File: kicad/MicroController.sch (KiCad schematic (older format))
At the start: 6 parts, among them P3 MIKROPROG, U1 LM324, U2 PIC16F1779

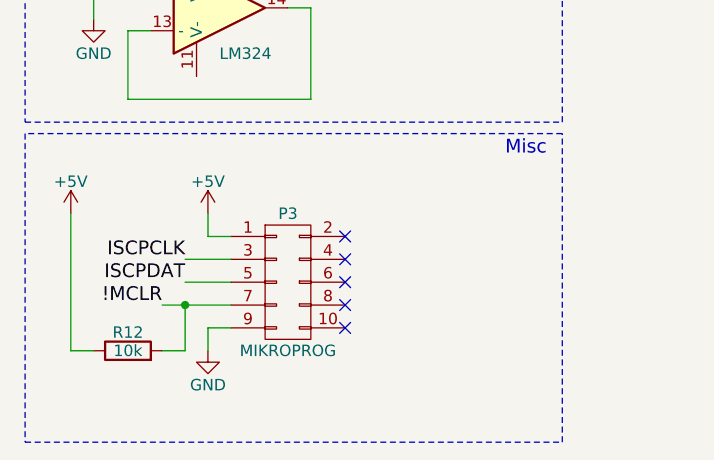
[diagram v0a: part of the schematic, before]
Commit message: Edited schematics
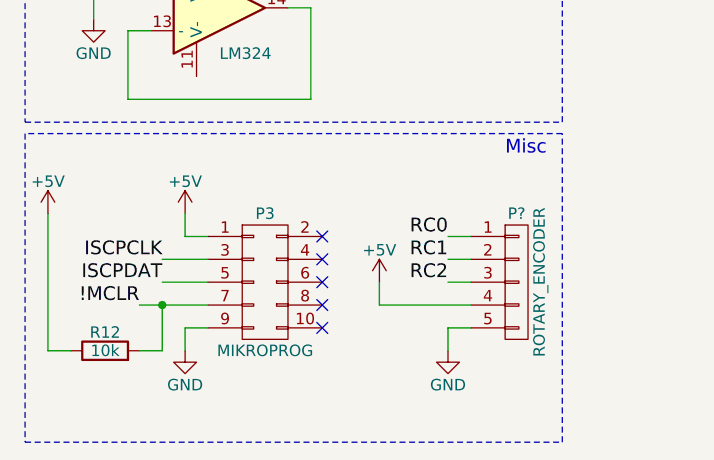
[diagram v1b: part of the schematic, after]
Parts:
- added P?: ROTARY_ENCODER, symbol CONN_01X05
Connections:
- net +5V: now also P?.4 (P4)
- net GND: now also P?.5 (P5)
- net RC0: now also P?.1 (P1)
- net RC1: now also P?.2 (P2)
- net RC2: now also P?.3 (P3)
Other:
- moved on the sheet: P3, R12
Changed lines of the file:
@@
 L CONN_02X05 P3
 U 1 1 59B71C9D
-P 1700 7000
-F 0 "P3" H 1700 7300 50  0000 C CNN
-F 1 "MIKROPROG" H 1700 6700 50  0000 C CNN
-F 2 "" H 1700 5800 50  0001 C CNN
-F 3 "" H 1700 5800 50  0000 C CNN
-	1    1700 7000
+P 1600 7000
+F 0 "P3" H 1600 7300 50  0000 C CNN
+F 1 "MIKROPROG" H 1600 6700 50  0000 C CNN
+F 2 "" H 1600 5800 50  0001 C CNN
+F 3 "" H 1600 5800 50  0000 C CNN
+	1    1600 7000
 	1    0    0    -1
 $EndComp
@@
 L +5V #PWR06
 U 1 1 59B71CA4
-P 750 6700
-F 0 "#PWR06" H 750 6550 50  0001 C CNN
-F 1 "+5V" H 750 6840 50  0000 C CNN
-F 2 "" H 750 6700 50  0000 C CNN
-F 3 "" H 750 6700 50  0000 C CNN
-	1    750  6700
-	1    0    0    -1
-$EndComp
-Wire Wire Line
-	1350 6700 1350 6800
-Wire Wire Line
-	1350 6800 1450 6800
-Text Label 1250 6900 2    60   ~ 0
+P 650 6700
+F 0 "#PWR06" H 650 6550 50  0001 C CNN
+F 1 "+5V" H 650 6840 50  0000 C CNN
+F 2 "" H 650 6700 50  0000 C CNN
+F 3 "" H 650 6700 50  0000 C CNN
+	1    650  6700
+	1    0    0    -1
+$EndComp
+Wire Wire Line
+	1250 6700 1250 6800
+Wire Wire Line
+	1250 6800 1350 6800
+Text Label 1150 6900 2    60   ~ 0
 ISCPCLK
-Text Label 1250 7000 2    60   ~ 0
+Text Label 1150 7000 2    60   ~ 0
 ISCPDAT
-Text Label 1150 7100 2    60   ~ 0
+Text Label 1050 7100 2    60   ~ 0
 !MCLR
 Wire Wire Line
-	1250 6900 1450 6900
-Wire Wire Line
-	1250 7000 1450 7000
-Wire Wire Line
-	1150 7100 1450 7100
-NoConn ~ 1950 6800
-NoConn ~ 1950 6900
-NoConn ~ 1950 7000
-NoConn ~ 1950 7100
-NoConn ~ 1950 7200
+	1150 6900 1350 6900
+Wire Wire Line
+	1150 7000 1350 7000
+Wire Wire Line
+	1050 7100 1350 7100
+NoConn ~ 1850 6800
+NoConn ~ 1850 6900
+NoConn ~ 1850 7000
+NoConn ~ 1850 7100
+NoConn ~ 1850 7200
 $Comp
 L GND #PWR07
 U 1 1 59B71CB7
-P 1350 7300
-F 0 "#PWR07" H 1350 7050 50  0001 C CNN
-F 1 "GND" H 1350 7150 50  0000 C CNN
-F 2 "" H 1350 7300 50  0000 C CNN
-F 3 "" H 1350 7300 50  0000 C CNN
-	1    1350 7300
-	1    0    0    -1
-$EndComp
-Wire Wire Line
-	1350 7200 1450 7200
+P 1250 7300
+F 0 "#PWR07" H 1250 7050 50  0001 C CNN
+F 1 "GND" H 1250 7150 50  0000 C CNN
+F 2 "" H 1250 7300 50  0000 C CNN
+F 3 "" H 1250 7300 50  0000 C CNN
+	1    1250 7300
+	1    0    0    -1
+$EndComp
+Wire Wire Line
+	1250 7200 1350 7200
 Text HLabel 1650 900  0    60   Input ~ 0
 5V
@@
 L R R12
 U 1 1 59B74780
-P 1000 7300
-F 0 "R12" V 1080 7300 50  0000 C CNN
-F 1 "10k" V 1000 7300 50  0000 C CNN
-F 2 "Resistors_SMD:R_0805_HandSoldering" V 930 7300 50  0001 C CNN
-F 3 "" H 1000 7300 50  0000 C CNN
-	1    1000 7300
+P 900 7300
+F 0 "R12" V 980 7300 50  0000 C CNN
+F 1 "10k" V 900 7300 50  0000 C CNN
+F 2 "Resistors_SMD:R_0805_HandSoldering" V 830 7300 50  0001 C CNN
+F 3 "" H 900 7300 50  0000 C CNN
+	1    900  7300
 	0    -1   -1   0
 $EndComp
 Wire Wire Line
-	1250 7100 1250 7300
-Connection ~ 1250 7100
+	1150 7100 1150 7300
+Connection ~ 1150 7100
 Wire Wire Line
 	1100 5100 1000 5100
@@
 	850  5700 1100 5700
 Wire Wire Line
-	1250 7300 1150 7300
-Wire Wire Line
-	850  7300 750  7300
-Wire Wire Line
-	750  7300 750  6700
+	1150 7300 1050 7300
+Wire Wire Line
+	750  7300 650  7300
+Wire Wire Line
+	650  7300 650  6700
 $Comp
 L +5V #PWR016
 U 1 1 59B75D07
-P 1350 6700
-F 0 "#PWR016" H 1350 6550 50  0001 C CNN
-F 1 "+5V" H 1350 6840 50  0000 C CNN
-F 2 "" H 1350 6700 50  0000 C CNN
-F 3 "" H 1350 6700 50  0000 C CNN
-	1    1350 6700
-	1    0    0    -1
-$EndComp
-Wire Wire Line
-	1350 7300 1350 7200
+P 1250 6700
+F 0 "#PWR016" H 1250 6550 50  0001 C CNN
+F 1 "+5V" H 1250 6840 50  0000 C CNN
+F 2 "" H 1250 6700 50  0000 C CNN
+F 3 "" H 1250 6700 50  0000 C CNN
+	1    1250 6700
+	1    0    0    -1
+$EndComp
+Wire Wire Line
+	1250 7300 1250 7200
 Wire Wire Line
 	3350 950  3250 950
@@
 Text Notes 4650 700  0    60   ~ 0
 MICROCONTROLLER
+$Comp
+L CONN_01X05 P?
+U 1 1 59B8D999
+P 2700 7000
+F 0 "P?" H 2700 7300 50  0000 C CNN
+F 1 "ROTARY_ENCODER" V 2800 7000 50  0000 C CNN
+F 2 "" H 2700 7000 50  0000 C CNN
+F 3 "" H 2700 7000 50  0000 C CNN
+	1    2700 7000
+	1    0    0    -1
+$EndComp
+$Comp
+L GND #PWR?
+U 1 1 59B8DA9A
+P 2400 7300
+F 0 "#PWR?" H 2400 7050 50  0001 C CNN
+F 1 "GND" H 2400 7150 50  0000 C CNN
+F 2 "" H 2400 7300 50  0000 C CNN
+F 3 "" H 2400 7300 50  0000 C CNN
+	1    2400 7300
+	1    0    0    -1
+$EndComp
+Wire Wire Line
+	2400 7300 2400 7200
+Wire Wire Line
+	2400 7200 2500 7200
+Text Label 2400 6800 2    60   ~ 0
+RC0
+Text Label 2400 6900 2    60   ~ 0
+RC1
+Text Label 2400 7000 2    60   ~ 0
+RC2
+Wire Wire Line
+	2400 6800 2500 6800
+Wire Wire Line
+	2400 6900 2500 6900
+Wire Wire Line
+	2400 7000 2500 7000
+$Comp
+L +5V #PWR?
+U 1 1 59B8E290
+P 2100 7000
+F 0 "#PWR?" H 2100 6850 50  0001 C CNN
+F 1 "+5V" H 2100 7140 50  0000 C CNN
+F 2 "" H 2100 7000 50  0000 C CNN
+F 3 "" H 2100 7000 50  0000 C CNN
+	1    2100 7000
+	1    0    0    -1
+$EndComp
+Wire Wire Line
+	2100 7000 2100 7100
+Wire Wire Line
+	2100 7100 2500 7100
 $EndSCHEMATC
